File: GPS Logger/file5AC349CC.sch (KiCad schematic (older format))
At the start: 23 parts, among them U6 APM4953, U7 APM4953

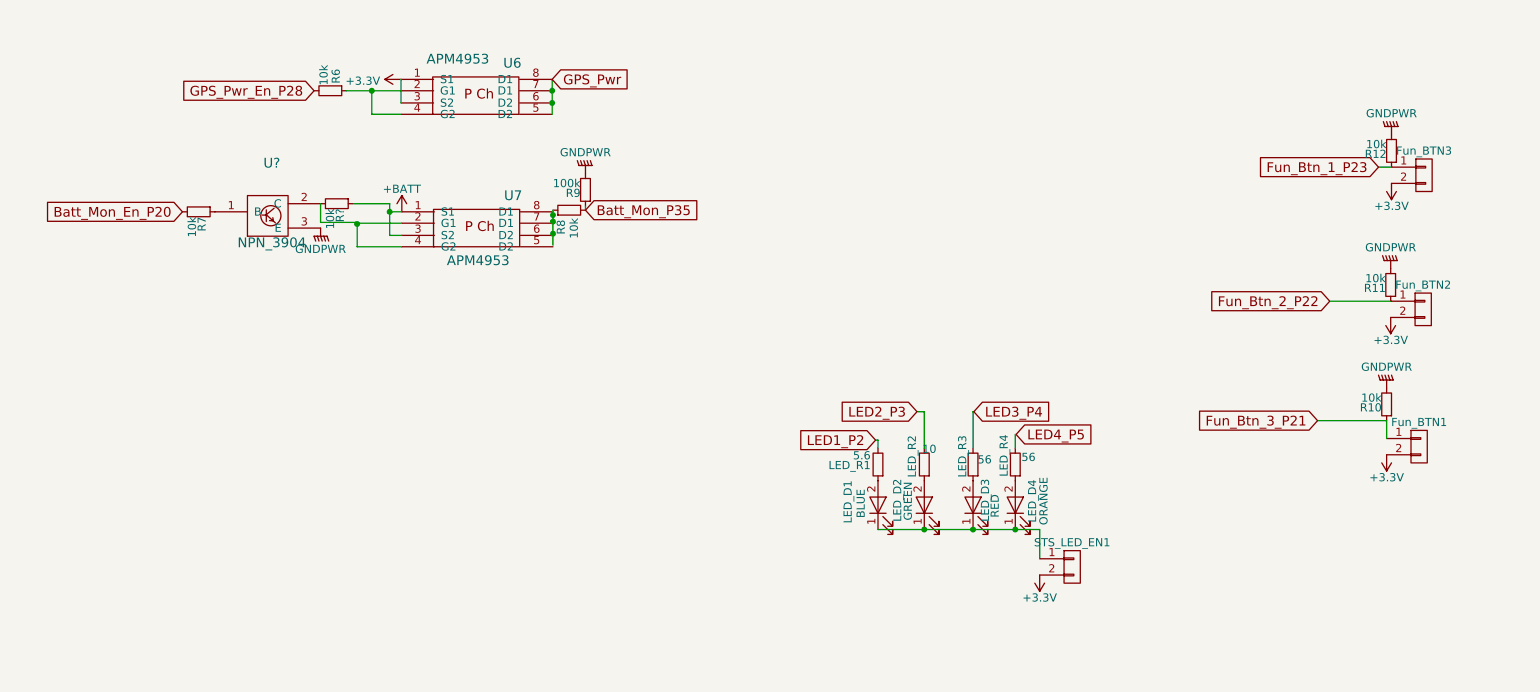
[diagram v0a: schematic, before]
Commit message: updated.  needs updates
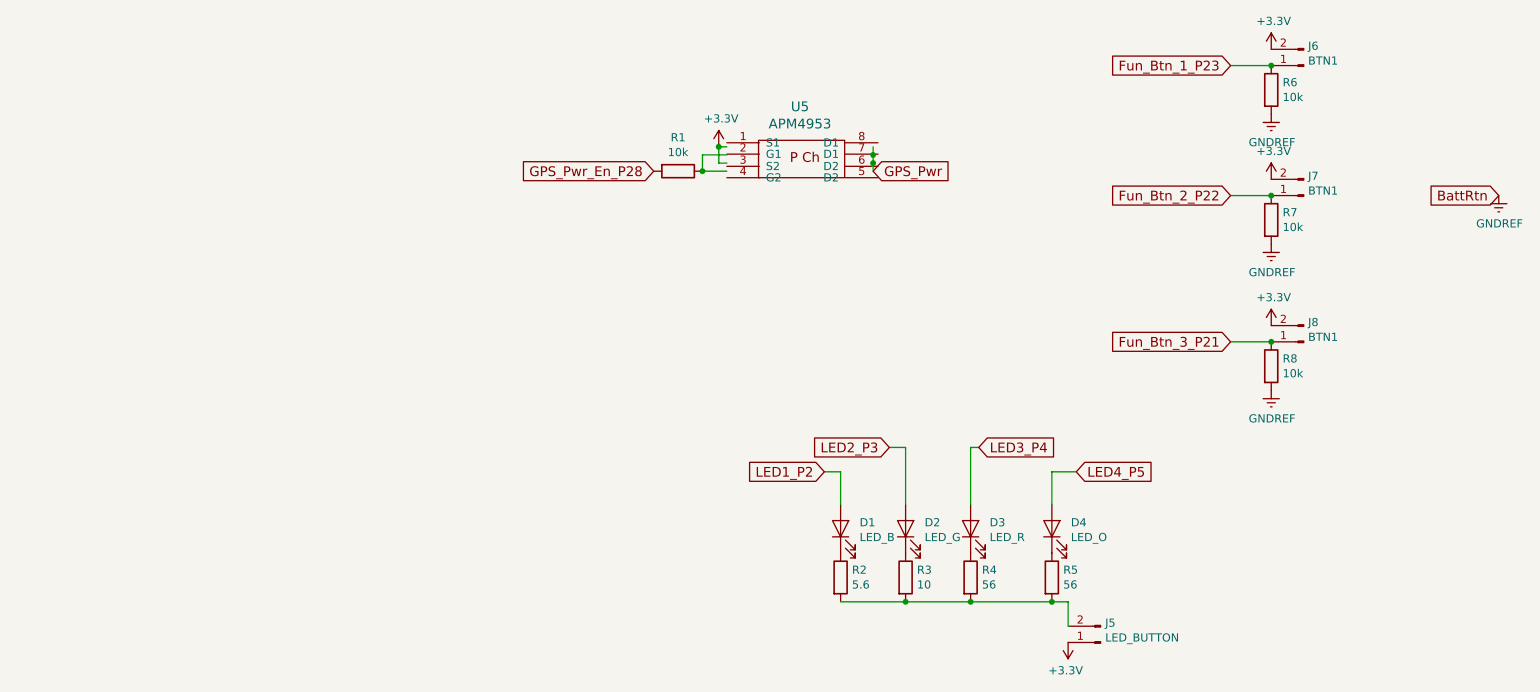
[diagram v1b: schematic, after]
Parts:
- removed Fun_BTN1: Fun_BTN, EbayParts:SMD_Switch_3x6, symbol CONN_01X02
- removed Fun_BTN2, Fun_BTN3: LVCutoff_reset, EbayParts:SMD_Switch_3x6, symbol CONN_01X02
- removed LED_D1: BLUE, LEDs:LED_0805, symbol LED
- removed LED_D2: GREEN, LEDs:LED_0805, symbol LED
- removed LED_D3: RED, LEDs:LED_0805, symbol LED
- removed LED_D4: ORANGE, LEDs:LED_0805, symbol LED
- removed LED_R1: 5.6, Resistors_SMD:R_0805_HandSoldering, symbol R_Small
- removed LED_R2: 10, Resistors_SMD:R_0805_HandSoldering, symbol R_Small
- removed LED_R3, LED_R4: 56, Resistors_SMD:R_0805_HandSoldering, symbol R_Small
- removed R10, R11, R12, R6, R7, R8, R?: 10k, Resistors_SMD:R_0805_HandSoldering, symbol R_Small
- removed R9: 100k, Resistors_SMD:R_0805_HandSoldering, symbol R_Small
- removed STS_LED_EN1: STS_LED_EN, EbayParts:SMD_Switch_3x6, symbol CONN_01X02
- removed U6, U7: APM4953, Housings_SOIC:SOIC-8_3.9x4.9mm_Pitch1.27mm, symbol APM4953
- removed U?: NPN_3904, symbol NPN_3904
- added D1: LED_B, LEDs:LED_0805, symbol Device:LED
- added D2: LED_G, LEDs:LED_0805, symbol Device:LED
- added D3: LED_R, LEDs:LED_0805, symbol Device:LED
- added D4: LED_O, LEDs:LED_0805, symbol Device:LED
- added J5: LED_BUTTON, EbayParts:Tact_SMD_Switch, symbol Connector:Conn_01x02_Male
- added J6, J7, J8: BTN1, EbayParts:Tact_SMD_Switch, symbol Connector:Conn_01x02_Male
- added R1, R6, R7, R8: 10k, Resistors_SMD:R_0805, symbol Device:R
- added R2: 5.6, Resistors_SMD:R_0805, symbol Device:R
- added R3: 10, Resistors_SMD:R_0805, symbol Device:R
- added R4, R5: 56, Resistors_SMD:R_0805, symbol Device:R
- added U5: APM4953, EbayParts:SOIC-8-N, symbol EbayParts:APM4953
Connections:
- net labels added: BattRtn, GNDREF
- net labels removed: +BATT, Batt_Mon_En_P20, Batt_Mon_P35, GNDPWR
- wire segments 31 -> 25
